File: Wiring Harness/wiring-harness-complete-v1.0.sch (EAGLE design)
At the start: 36 parts, among them J1 M80-879, J10 SMA-142-0701-801/806, J11 SMA-142-0701-801/806, J12 SMA-142-0701-801/806, J13 SMA-142-0701-801/806, J16 SMA-142-0701-801/806, J17 SMA-142-0701-801/806, J18 SMA-142-0701-871/880, J19 SMA-142-0701-871/880, J2 M80-5000000M1-10-331-000, J20 GLENAIR-171-006-6-S-6-7-18, J21 GLENAIR-171-006-6-S-6-7-18, J22 GLENAIR-171-006-6-S-6-7-18, J23 GLENAIR-171-006-6-S-6-7-18, J3 M80-5000000M1-10-331-00-000, J30 M80-866XXXX, J31 M80-866XXXX, J4 SMFC, J50 22-27-2021-02, J53 22-05-7028-02, SW1 CT10-XXXX-A2, SW2 CT10-XXXX-A2, SW3 CT10-XXXX-A2, X16 5566-14

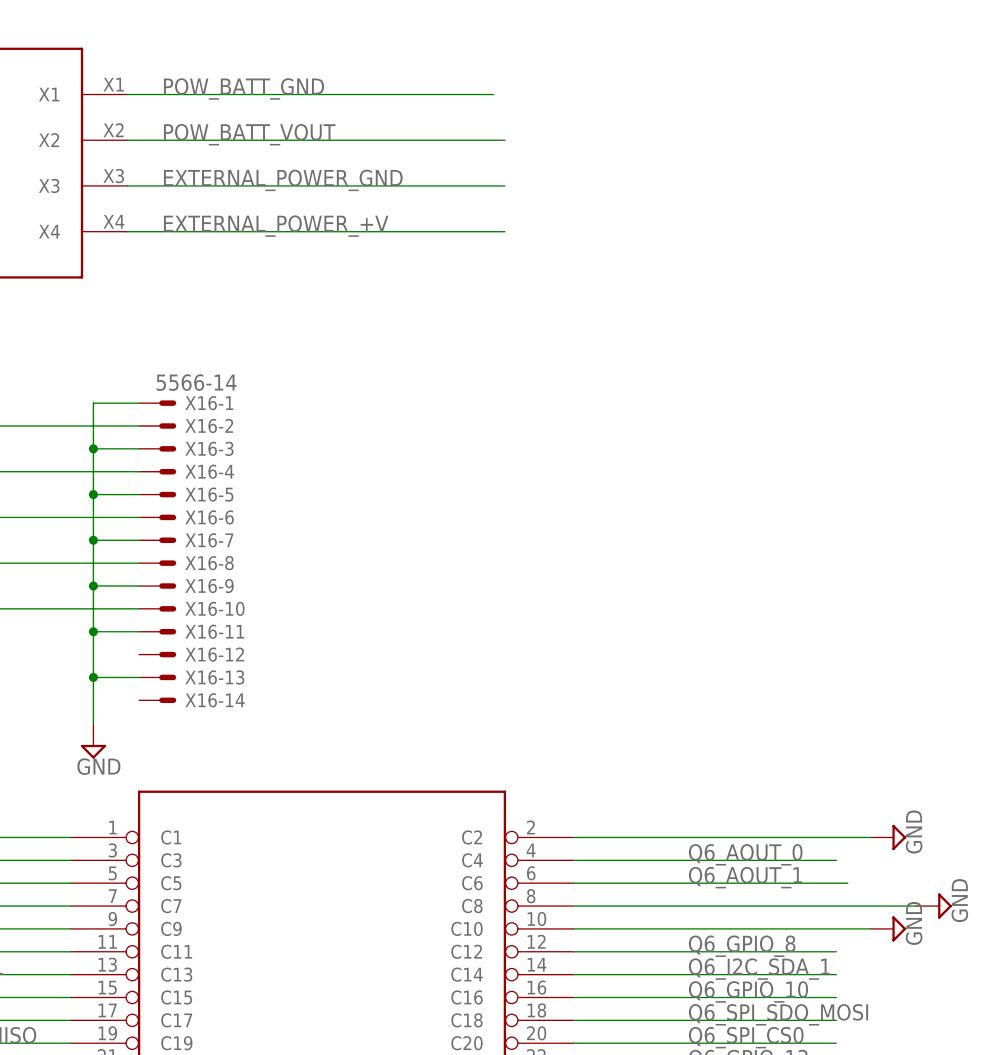
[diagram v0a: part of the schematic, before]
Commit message: [CDH] - fixed typos in signal netnames so they match wiring-harness   - updated 'EXTERNAL_POWER_+V' and 'EXTERNAL_POWER_GND' so that they match the EPS header [WIRING] - updated 'EXTERNAL_POWER_+V' and 'EXTERNAL_POWER_GND' so that they properly route through the wiring harness
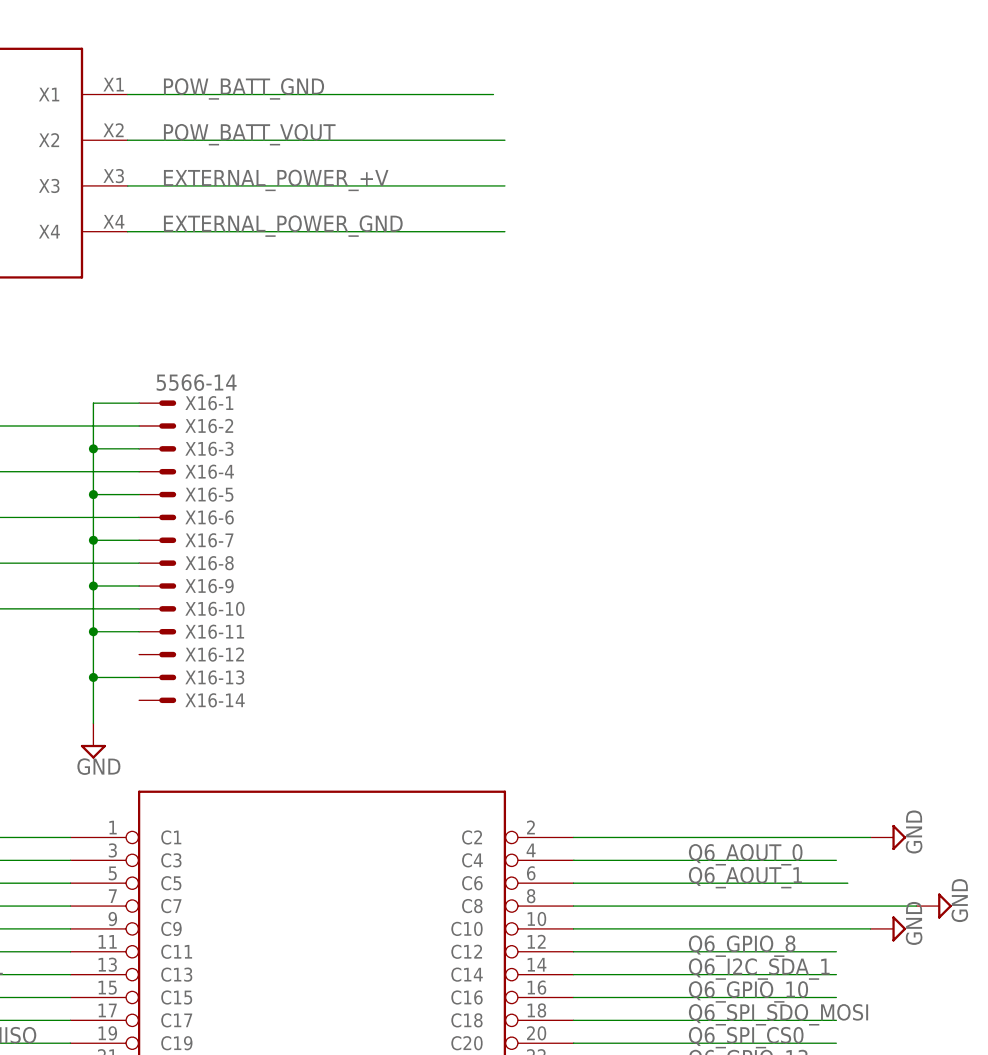
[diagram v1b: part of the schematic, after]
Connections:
- removed net Q6_AOUT_2: J4.C4
- removed net Q6_AOUT_3: J4.C6
- net EXTERNAL_POWER_+V: now also J3.X3; no longer J3.X4
- net EXTERNAL_POWER_GND: now also J3.X4; no longer J3.X3
- net Q6_AOUT_0: now also J4.C4
- net Q6_AOUT_1: now also J4.C6
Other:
- note removed: "Q6_AOUT_0"
- note removed: "Q6_AOUT_1"
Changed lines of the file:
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@@
 <setting verticaltext="up"/>
 </settings>
-<grid distance="1.27" unitdist="mm" unit="mm" style="lines" multiple="1" display="no" altdistance="0.01" altunitdist="inch" altunit="mm"/>
+<grid distance="0.1" unitdist="inch" unit="inch" style="lines" multiple="1" display="no" altdistance="0.01" altunitdist="inch" altunit="inch"/>
 <layers>
 <layer number="1" name="Top" color="4" fill="1" visible="no" active="no"/>
@@
 <text x="17.78" y="-45.72" size="1.778" layer="95">SOLAR_PANEL_2_4</text>
 <text x="35.46" y="-93.59" size="1.778" layer="95">3V3_CTL</text>
-<text x="35.56" y="124.46" size="1.778" layer="95">Q6_AOUT_0</text>
-<text x="35.56" y="121.92" size="1.778" layer="95">Q6_AOUT_1</text>
 <text x="-15.24" y="88.9" size="2.1844" layer="95">Q6-Connector</text>
 <wire x1="-200.66" y1="284.48" x2="93.98" y2="284.48" width="0.1524" layer="152" style="longdash"/>
@@
 <label x="-53.34" y="-193.04" size="1.778" layer="95"/>
 </segment>
+<segment>
+<wire x1="22.86" y1="124.46" x2="52.07" y2="124.46" width="0.1524" layer="91"/>
+<pinref part="J4" gate="G$1" pin="C4"/>
+<label x="35.56" y="124.46" size="1.778" layer="95"/>
+</segment>
 </net>
 <net name="Q6_AOUT_1" class="0">
@@
 <wire x1="-15.24" y1="-109.22" x2="-43.18" y2="-109.22" width="0.1524" layer="91"/>
 <label x="-40.64" y="-109.22" size="1.778" layer="95"/>
+</segment>
+<segment>
+<wire x1="22.86" y1="121.92" x2="53.34" y2="121.92" width="0.1524" layer="91"/>
+<pinref part="J4" gate="G$1" pin="C6"/>
+<label x="35.56" y="121.92" size="1.778" layer="95"/>
 </segment>
 </net>
@@
 </segment>
 <segment>
-<pinref part="J3" gate="G$1" pin="X4"/>
-<wire x1="-26.67" y1="194.31" x2="15.24" y2="194.31" width="0.1524" layer="91"/>
-<label x="-22.86" y="194.31" size="1.778" layer="95"/>
-</segment>
-<segment>
 <wire x1="-317.5" y1="215.9" x2="-281.94" y2="215.9" width="0.1524" layer="91"/>
 <label x="-304.8" y="215.9" size="1.778" layer="95"/>
@@
 <segment>
 <wire x1="-414.02" y1="218.44" x2="-386.08" y2="218.44" width="0.1524" layer="91"/>
+</segment>
+<segment>
+<pinref part="J3" gate="G$1" pin="X3"/>
+<wire x1="-26.67" y1="199.39" x2="15.24" y2="199.39" width="0.1524" layer="91"/>
+<label x="-22.86" y="199.39" size="1.778" layer="95"/>
 </segment>
 </net>
@@
 </segment>
 <segment>
-<pinref part="J3" gate="G$1" pin="X3"/>
-<wire x1="-26.67" y1="199.39" x2="15.24" y2="199.39" width="0.1524" layer="91"/>
-<label x="-22.86" y="199.39" size="1.778" layer="95"/>
-</segment>
-<segment>
 <wire x1="-281.94" y1="218.44" x2="-317.5" y2="218.44" width="0.1524" layer="91"/>
 <label x="-304.8" y="218.44" size="1.778" layer="95"/>
@@
 <wire x1="-429.26" y1="218.44" x2="-468.63" y2="218.44" width="0.1524" layer="91"/>
 </segment>
+<segment>
+<pinref part="J3" gate="G$1" pin="X4"/>
+<wire x1="-26.67" y1="194.31" x2="15.24" y2="194.31" width="0.1524" layer="91"/>
+<label x="-22.86" y="194.31" size="1.778" layer="95"/>
+</segment>
 </net>
 <net name="POW_9V" class="0">
@@
 </segment>
 </net>
-<net name="Q6_AOUT_2" class="0">
-<segment>
-<wire x1="22.86" y1="124.46" x2="52.07" y2="124.46" width="0.1524" layer="91"/>
-<pinref part="J4" gate="G$1" pin="C4"/>
-</segment>
-</net>
-<net name="Q6_AOUT_3" class="0">
-<segment>
-<wire x1="22.86" y1="121.92" x2="53.34" y2="121.92" width="0.1524" layer="91"/>
-<pinref part="J4" gate="G$1" pin="C6"/>
-</segment>
-</net>

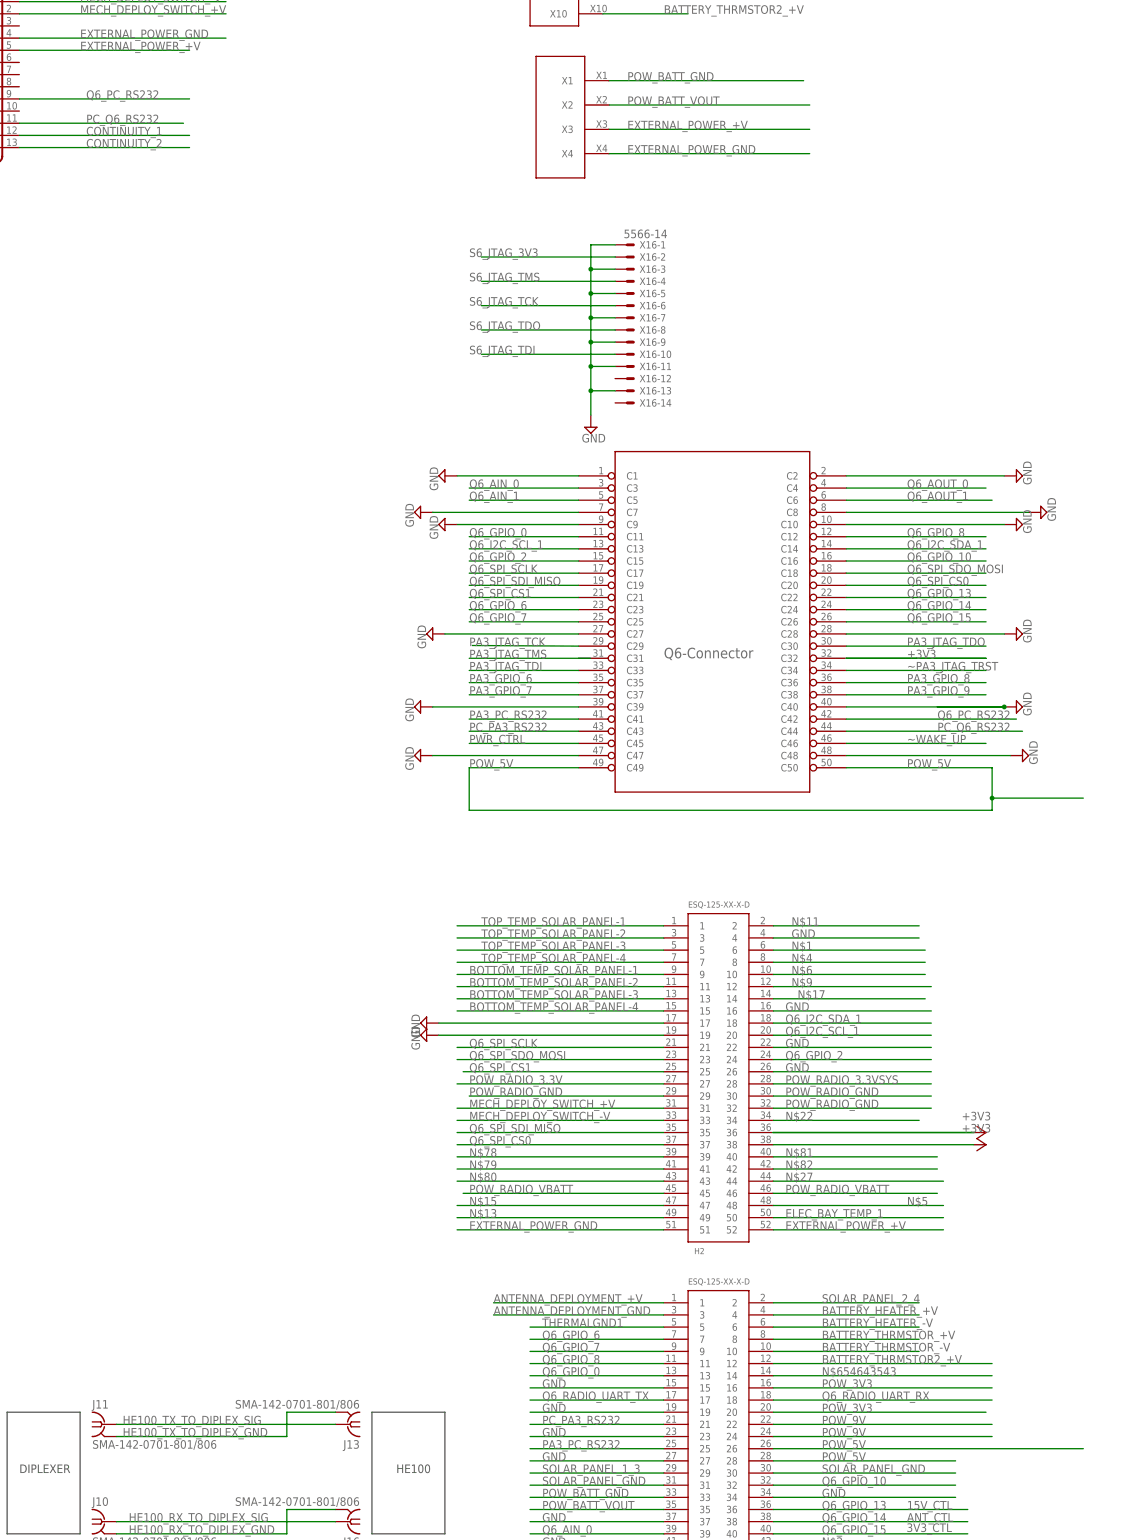
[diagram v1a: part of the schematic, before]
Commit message: [CDH] [Wiring Harness] [Payload-Internal-Aux] renamed nets 'Q6_PC_RS232' and 'PC_Q6_RS232' to 'Q6_MAX_RS232' and 'MAX_Q6_RS232' for clarity
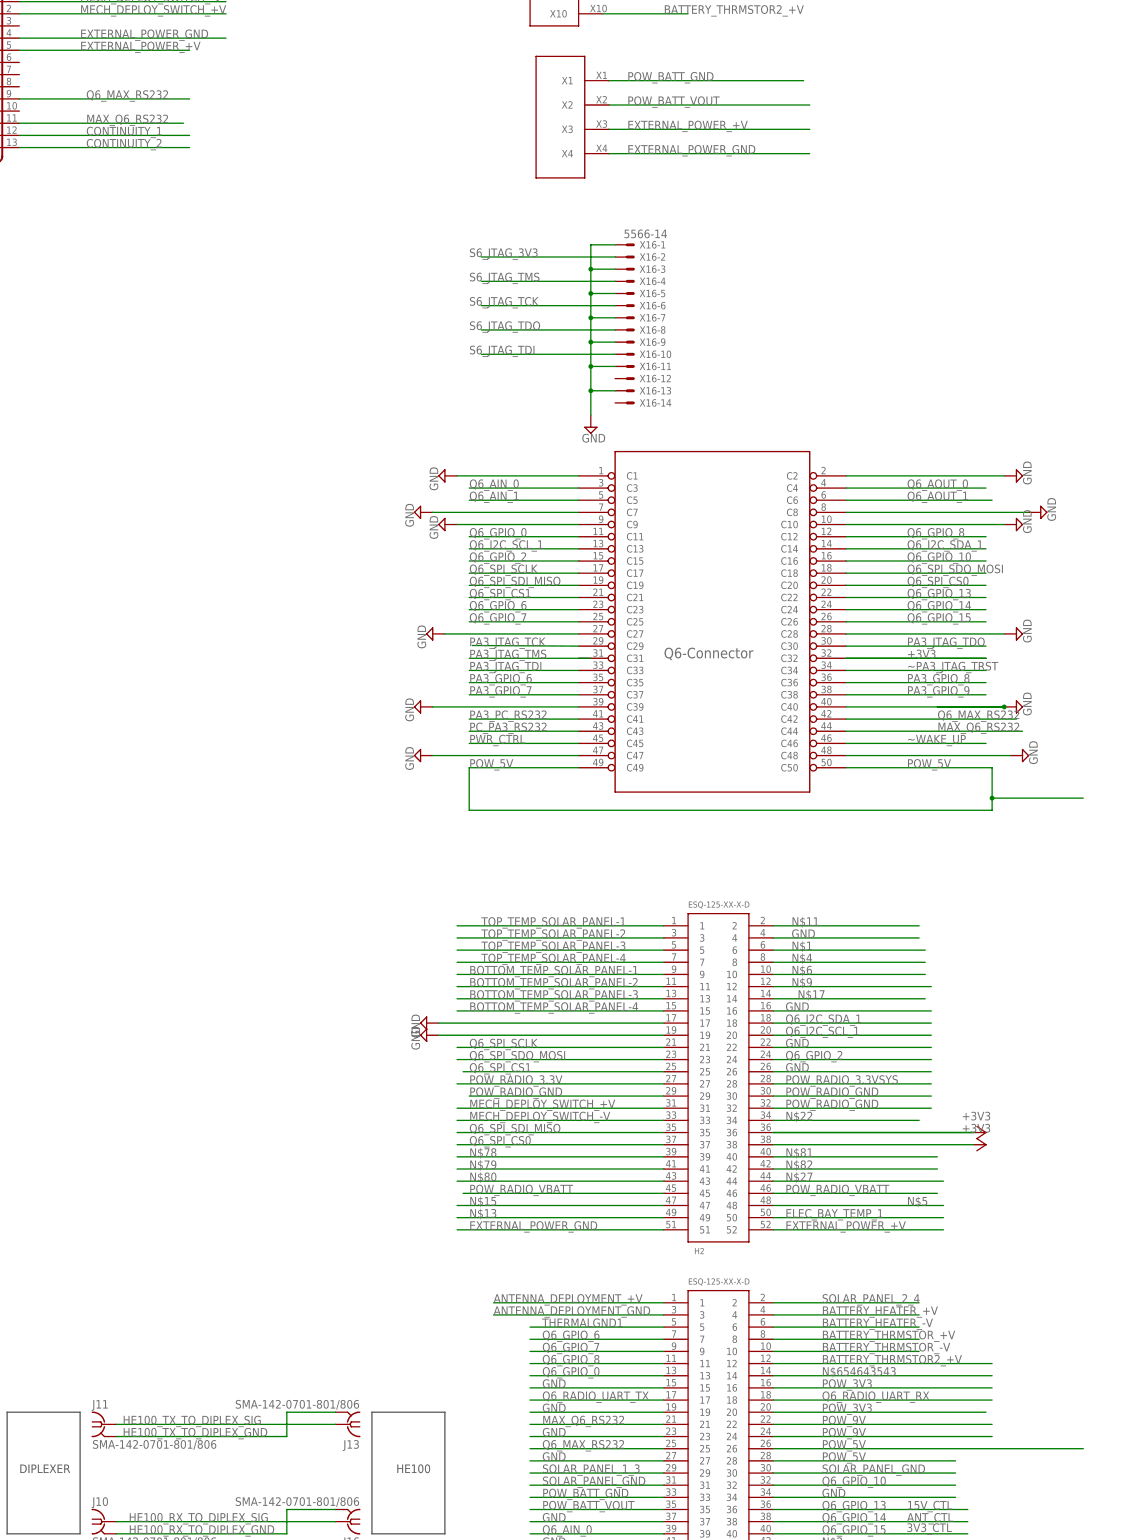
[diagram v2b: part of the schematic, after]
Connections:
- removed net PC_Q6_RS232: J4.C44
- removed net Q6_PC_RS232: J4.C42
- new net MAX_Q6_RS232: H1.21, J4.C44
- new net Q6_MAX_RS232: H1.25, J4.C42
- net PA3_PC_RS232: no longer H1.25
- net PC_PA3_RS232: no longer H1.21
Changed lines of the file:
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@@
 <net name="PC_PA3_RS232" class="0">
-<segment>
-<pinref part="H1" gate="G$1" pin="21"/>
-<wire x1="-15.24" y1="-71.12" x2="-43.18" y2="-71.12" width="0.1524" layer="91"/>
-<label x="-40.64" y="-71.12" size="1.778" layer="95"/>
-</segment>
 <segment>
 <pinref part="J4" gate="G$1" pin="C43"/>
@@
 </net>
 <net name="PA3_PC_RS232" class="0">
-<segment>
-<pinref part="H1" gate="G$1" pin="25"/>
-<wire x1="-15.24" y1="-76.2" x2="-43.18" y2="-76.2" width="0.1524" layer="91"/>
-<label x="-40.64" y="-76.2" size="1.778" layer="95"/>
-</segment>
 <segment>
 <pinref part="J4" gate="G$1" pin="C41"/>
@@
 <net name="Q6_PC_RS232" class="0">
 <segment>
-<pinref part="J4" gate="G$1" pin="C42"/>
-<wire x1="22.86" y1="76.2" x2="58.42" y2="76.2" width="0.1524" layer="91"/>
-<label x="41.91" y="76.2" size="1.778" layer="95"/>
-<label x="-135.89" y="205.74" size="1.778" layer="95"/>
-</segment>
-<segment>
 <label x="-303.53" y="205.74" size="1.778" layer="95"/>
 <label x="-394.97" y="220.98" size="1.778" layer="95"/>
@@
 </net>
 <net name="PC_Q6_RS232" class="0">
-<segment>
-<pinref part="J4" gate="G$1" pin="C44"/>
-<label x="41.91" y="73.66" size="1.778" layer="95"/>
-<wire x1="22.86" y1="73.66" x2="59.69" y2="73.66" width="0.1524" layer="91"/>
-<label x="-135.89" y="200.66" size="1.778" layer="95"/>
-</segment>
 <segment>
 <label x="-303.53" y="200.66" size="1.778" layer="95"/>
@@
 </segment>
 </net>
+<net name="Q6_MAX_RS232" class="0">
+<segment>
+<pinref part="H1" gate="G$1" pin="25"/>
+<wire x1="-15.24" y1="-76.2" x2="-43.18" y2="-76.2" width="0.1524" layer="91"/>
+<label x="-40.64" y="-76.2" size="1.778" layer="95"/>
+</segment>
+<segment>
+<pinref part="J4" gate="G$1" pin="C42"/>
+<wire x1="22.86" y1="76.2" x2="58.42" y2="76.2" width="0.1524" layer="91"/>
+<label x="41.91" y="76.2" size="1.778" layer="95"/>
+<label x="-135.89" y="205.74" size="1.778" layer="95"/>
+</segment>
+</net>
+<net name="MAX_Q6_RS232" class="0">
+<segment>
+<pinref part="H1" gate="G$1" pin="21"/>
+<wire x1="-15.24" y1="-71.12" x2="-43.18" y2="-71.12" width="0.1524" layer="91"/>
+<label x="-40.64" y="-71.12" size="1.778" layer="95"/>
+</segment>
+<segment>
+<pinref part="J4" gate="G$1" pin="C44"/>
+<label x="41.91" y="73.66" size="1.778" layer="95"/>
+<wire x1="22.86" y1="73.66" x2="59.69" y2="73.66" width="0.1524" layer="91"/>
+<label x="-135.89" y="200.66" size="1.778" layer="95"/>
+</segment>
+</net>
